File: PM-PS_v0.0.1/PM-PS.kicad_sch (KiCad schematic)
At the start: 18 parts, among them J2 PinHeader_01x05_P2.54_THT_ang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, J3 2EDGR-5.08-10P, J4 K7805-2000R3, J5 K7803-2000R3, U1 IRM-20-24, U2 64900001039, U3 64900001039, U4 64900001039

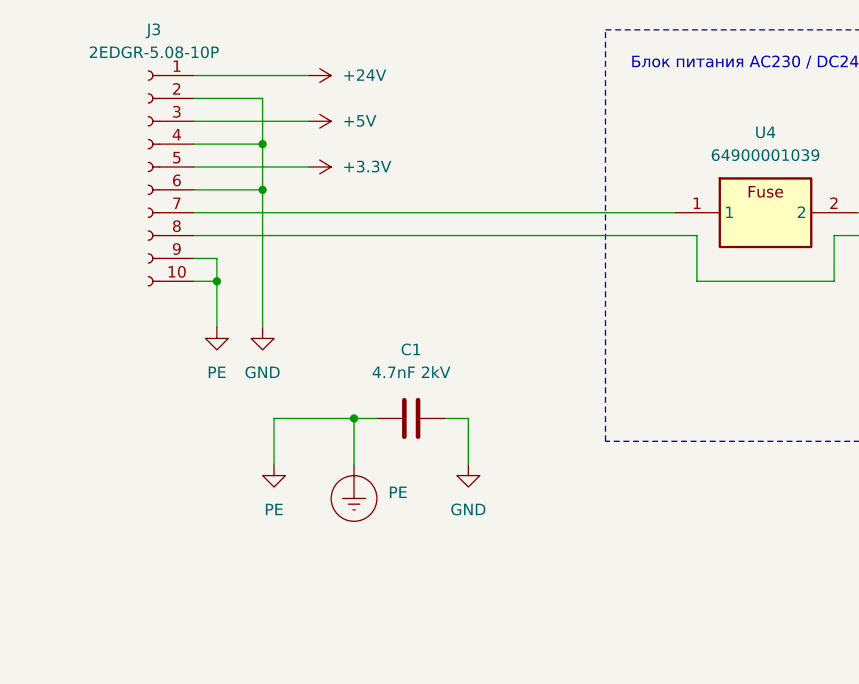
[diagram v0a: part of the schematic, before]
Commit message: create firmware project
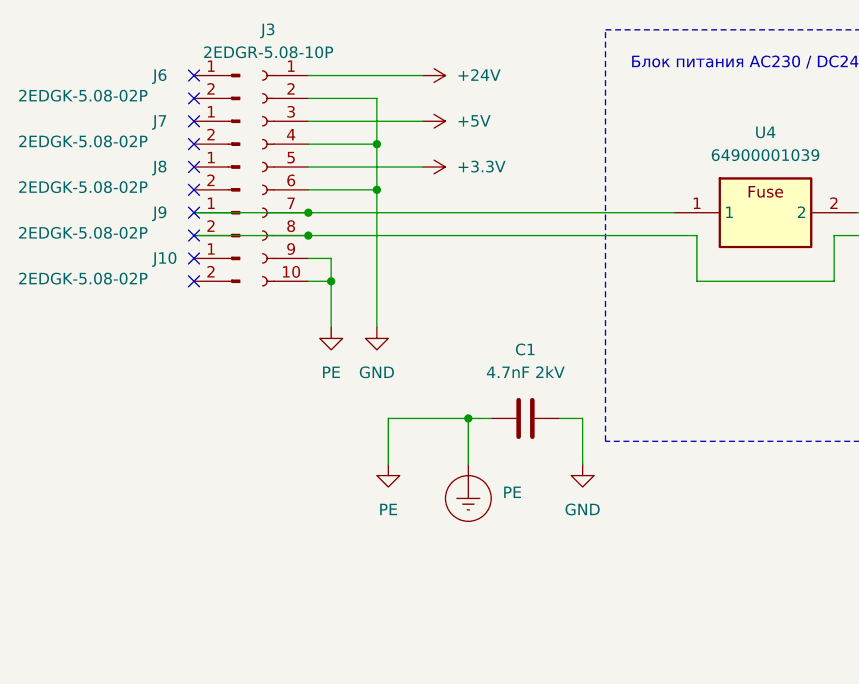
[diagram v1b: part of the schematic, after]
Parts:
- added J10, J6, J7, J8, J9: 2EDGK-5.08-02P, symbol kicad_inventree_lib:Degson_2EDGK-5.08-02P
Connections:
- net N: now also J9.2 (Pin_2)
- net at J3.7 (Pin_7), U4.1: now also J9.1 (Pin_1)
- no-connect marks 2 -> 12
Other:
- moved on the sheet: C1, J3
